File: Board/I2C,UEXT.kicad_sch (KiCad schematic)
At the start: 7 parts, among them IC24 PCF9564, J7 UEXT_Host

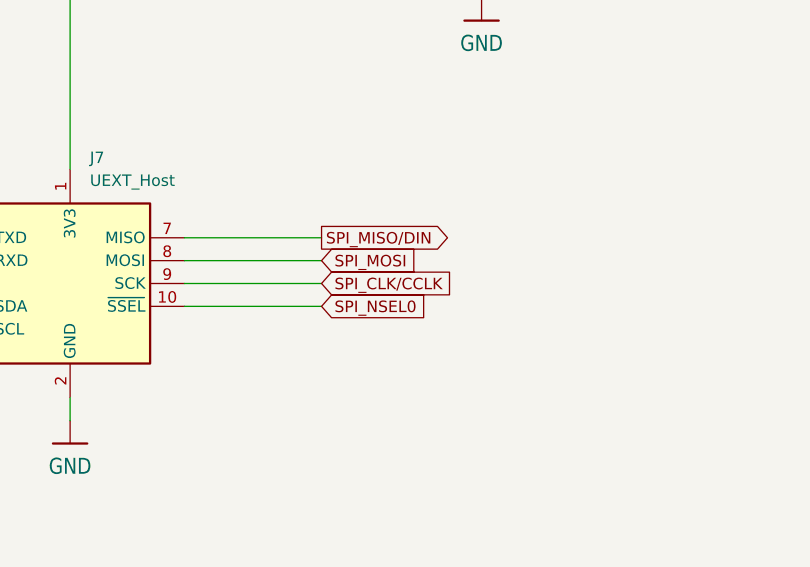
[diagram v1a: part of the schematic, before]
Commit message: more work on 1.3
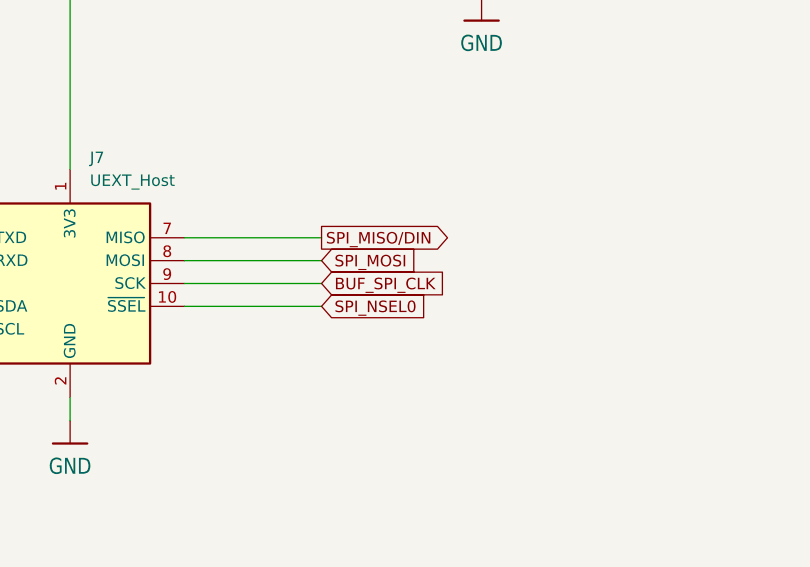
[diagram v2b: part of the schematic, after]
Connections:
- net SPI_CLK/CCLK renamed BUF_SPI_CLK
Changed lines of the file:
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@@
-		)
-	)
-	(global_label "SPI_CLK{slash}CCLK"
-		(shape input)
-		(at 196.85 105.41 0)
-		(fields_autoplaced yes)
-		(effects
-			(font
-				(size 1.27 1.27)
-			)
-			(justify left)
-		)
-		(property "Intersheetrefs" "${INTERSHEET_REFS}"
-			(at 213.6238 105.41 0)
-			(effects
-				(font
-					(size 1.27 1.27)
-				)
-				(justify left)
-				(hide yes)
-			)
 		)
 	)
@@
 				(hide yes)
 			)
+		)
+	)
+	(global_label "BUF_SPI_CLK"
+		(shape input)
+		(at 196.85 105.41 0)
+		(fields_autoplaced yes)
+		(effects
+			(font
+				(size 1.27 1.27)
+			)
+			(justify left)
+		)
+		(property "Intersheetrefs" "${INTERSHEET_REFS}"
+			(at 212.1119 105.41 0)
+			(effects
+				(font
+					(size 1.27 1.27)
+				)
+				(justify left)
+				(hide yes)
+			)

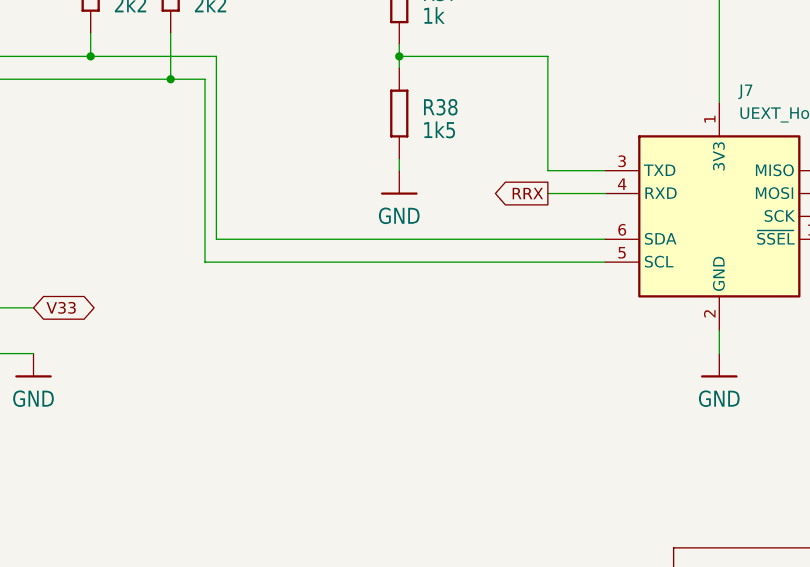
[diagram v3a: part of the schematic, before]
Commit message: more work on r1.3
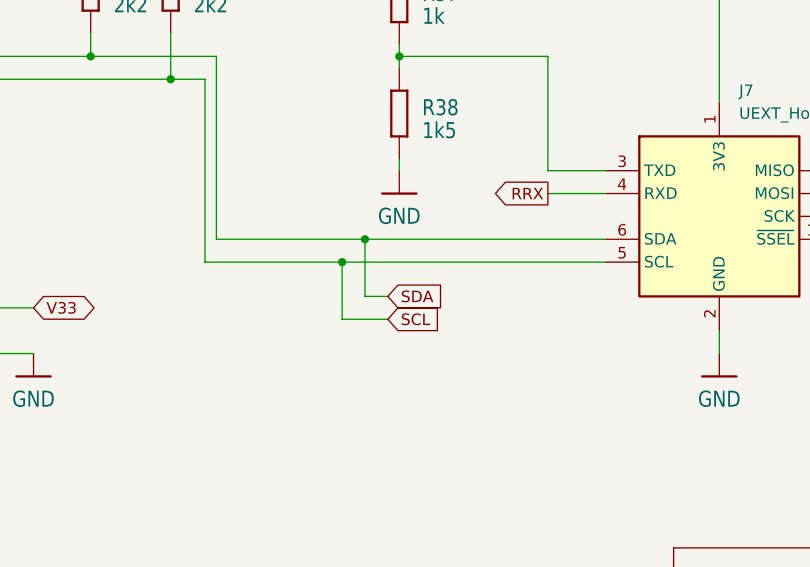
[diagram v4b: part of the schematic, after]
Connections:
- net SCL: now reaches IC24.18 (SCL), J7.5 (SCL), R36.2
- net SDA: now reaches IC24.19 (SDA), J7.6 (SDA), R23.2
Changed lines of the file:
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@@
+	)
+	(junction
+		(at 127 110.49)
+		(diameter 0)
+		(color 0 0 0 0)
+	)
+	(junction
+		(at 129.54 107.95)
+		(diameter 0)
+		(color 0 0 0 0)
 	)
 	(junction
@@
 	(wire
 		(pts
+			(xy 127 110.49) (xy 156.21 110.49)
+		)
+		(stroke
+			(width 0)
+			(type default)
+		)
+	)
+	(wire
+		(pts
 			(xy 99.06 85.09) (xy 99.06 87.63)
 		)
@@
 	(wire
 		(pts
+			(xy 132.08 114.3) (xy 129.54 114.3)
+		)
+		(stroke
+			(width 0)
+			(type default)
+		)
+	)
+	(wire
+		(pts
 			(xy 48.26 99.06) (xy 64.77 99.06)
 		)
@@
 	(wire
 		(pts
+			(xy 129.54 114.3) (xy 129.54 107.95)
+		)
+		(stroke
+			(width 0)
+			(type default)
+		)
+	)
+	(wire
+		(pts
 			(xy 48.26 101.6) (xy 64.77 101.6)
 		)
@@
 	(wire
 		(pts
-			(xy 111.76 110.49) (xy 156.21 110.49)
+			(xy 111.76 110.49) (xy 127 110.49)
 		)
 		(stroke
@@
 	(wire
 		(pts
+			(xy 127 116.84) (xy 127 110.49)
+		)
+		(stroke
+			(width 0)
+			(type default)
+		)
+	)
+	(wire
+		(pts
 			(xy 48.26 96.52) (xy 64.77 96.52)
 		)
@@
 	(wire
 		(pts
+			(xy 132.08 116.84) (xy 127 116.84)
+		)
+		(stroke
+			(width 0)
+			(type default)
+		)
+	)
+	(wire
+		(pts
 			(xy 48.26 132.08) (xy 64.77 132.08)
 		)
@@
 	(wire
 		(pts
-			(xy 113.03 107.95) (xy 156.21 107.95)
+			(xy 113.03 107.95) (xy 129.54 107.95)
 		)
 		(stroke
@@
 		(pts
 			(xy 107.95 90.17) (xy 111.76 90.17)
+		)
+		(stroke
+			(width 0)
+			(type default)
+		)
+	)
+	(wire
+		(pts
+			(xy 129.54 107.95) (xy 156.21 107.95)
 		)
 		(stroke
@@
 		)
 	)
+	(global_label "SDA"
+		(shape input)
+		(at 132.08 114.3 0)
+		(fields_autoplaced yes)
+		(effects
+			(font
+				(size 1.27 1.27)
+			)
+			(justify left)
+		)
+		(property "Intersheetrefs" "${INTERSHEET_REFS}"
+			(at 138.6333 114.3 0)
+			(effects
+				(font
+					(size 1.27 1.27)
+				)
+				(justify left)
+				(hide yes)
+			)
+		)
+	)
 	(global_label "BUF_SPI_CLK"
 		(shape input)
@@
 				(hide yes)
 			)
+		)
+	)
+	(global_label "SCL"
+		(shape input)
+		(at 132.08 116.84 0)
+		(fields_autoplaced yes)
+		(effects
+			(font
+				(size 1.27 1.27)
+			)
+			(justify left)
+		)
+		(property "Intersheetrefs" "${INTERSHEET_REFS}"
+			(at 138.5728 116.84 0)
+			(effects
+				(font
+					(size 1.27 1.27)
+				)
+				(justify left)
+				(hide yes)
+			)
